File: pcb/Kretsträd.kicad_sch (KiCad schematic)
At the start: 56 parts, among them J1 Conn_01x02_Female, J2 Conn_01x02_Female, J3 Conn_01x02_Female, SW1 SW_PUSH, SW10 SW_PUSH, SW11 SW_PUSH, SW12 SW_PUSH, SW13 SW_PUSH, SW14 SW_PUSH, SW15 SW_PUSH, SW16 SW_PUSH, SW17 SW_PUSH, SW2 SW_PUSH, SW3 SW_PUSH, SW4 SW_PUSH, SW5 SW_PUSH, SW6 SW_PUSH, SW7 SW_PUSH, SW8 SW_PUSH, SW9 SW_PUSH, U1 SeeeduinoXIAO

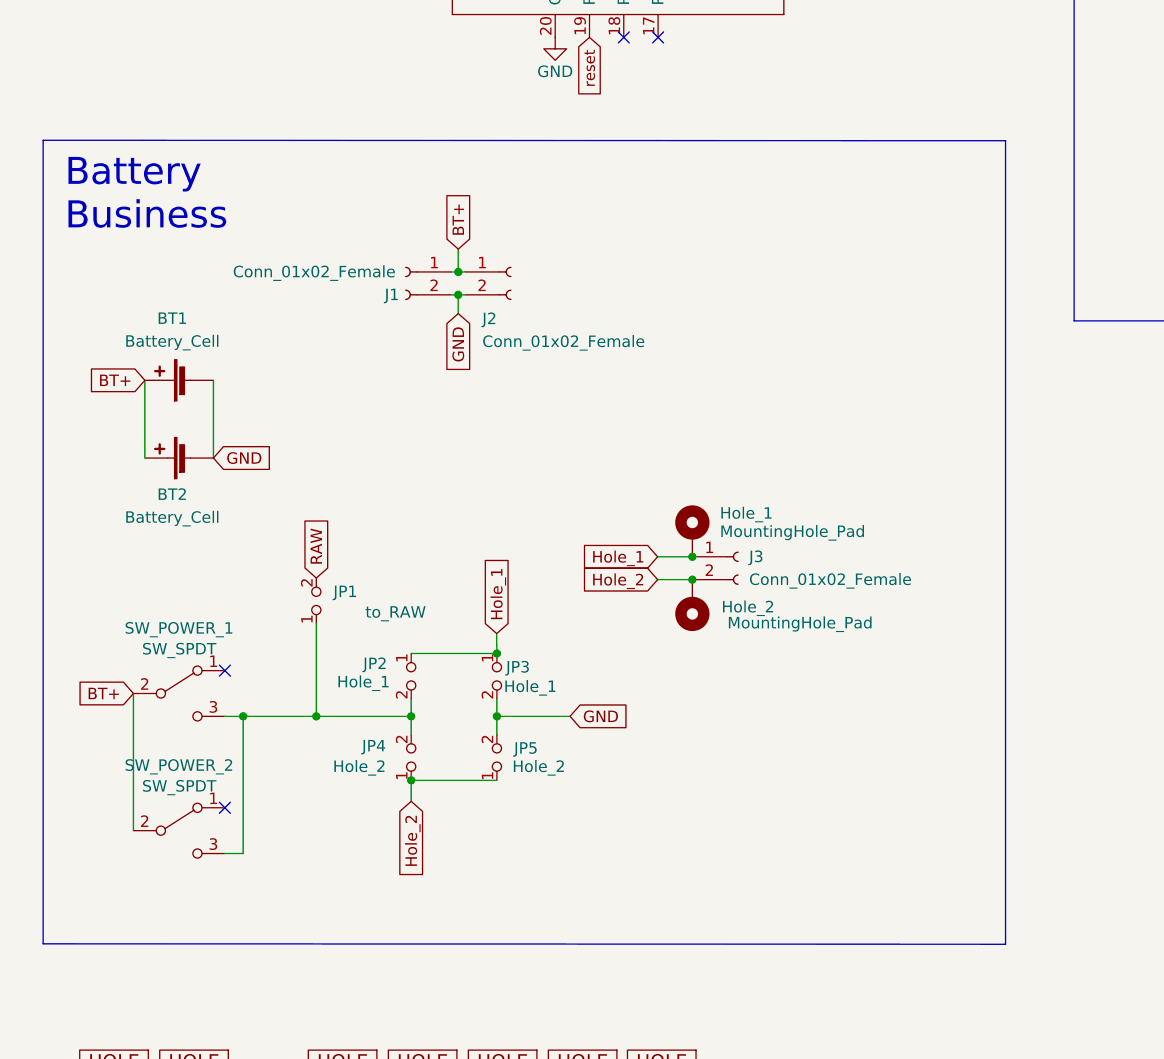
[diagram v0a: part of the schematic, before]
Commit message: Tones of changes.
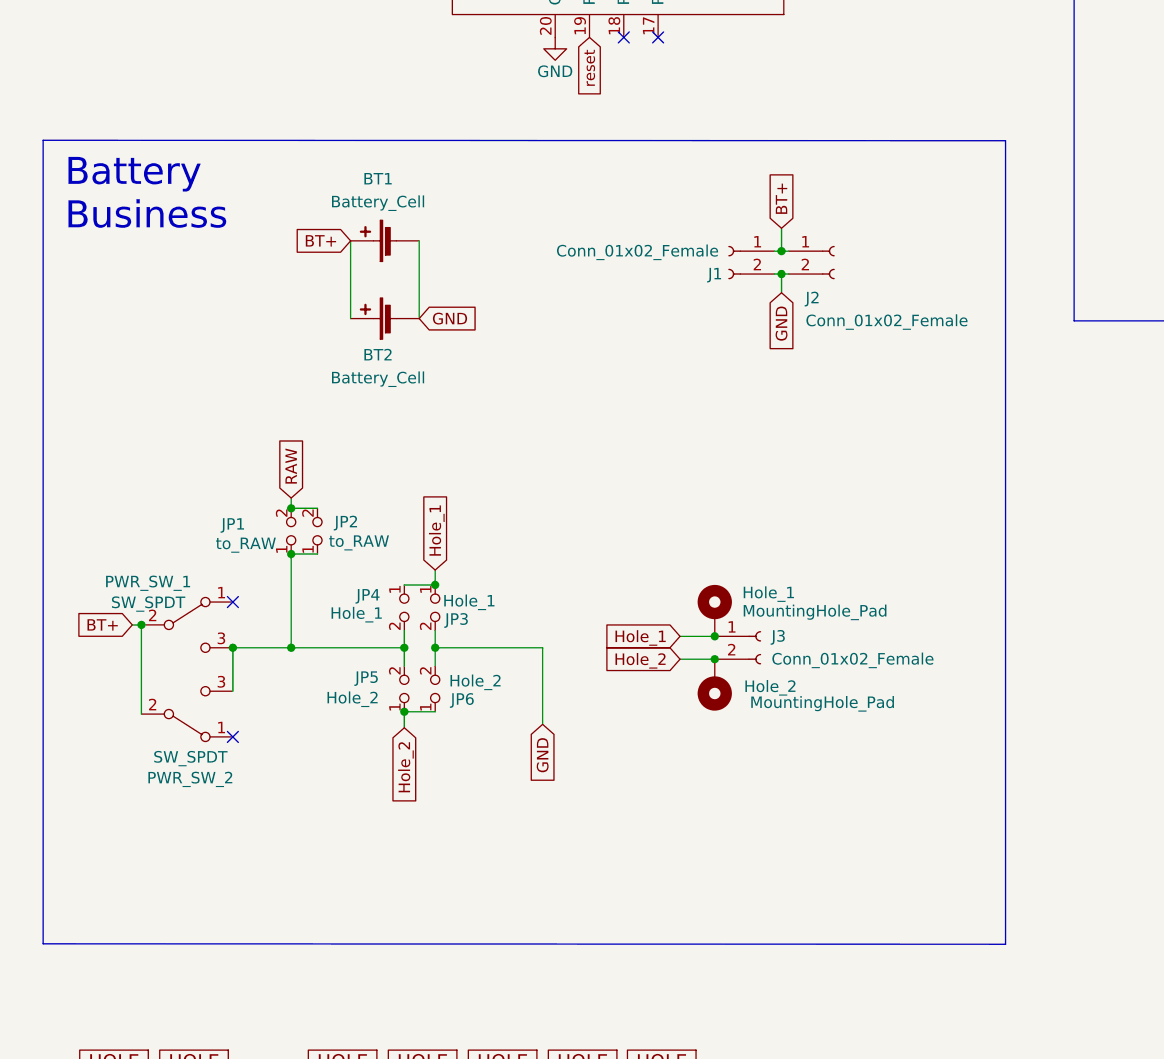
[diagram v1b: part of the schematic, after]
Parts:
- added JP1: to_RAW, Jumper:SolderJumper-2_P1.3mm_Open_RoundedPad1.0x1.5mm, symbol Device:Jumper_NO_Small
- D1, D10, D11, D12, D13, D14, D15, D16, D17, D2, D3, D4, D5, D6, D7, D8, D9: footprint jw_custom_footprint:D_SOD123_THT -> jw_custom_footprint:Diode_SOD123_THT_2
- JP2: renamed from JP1; footprint Jumper:SolderJumper-2_P1.3mm_Open_TrianglePad1.0x1.5mm -> Jumper:SolderJumper-2_P1.3mm_Open_RoundedPad1.0x1.5mm
- JP3: renamed from JP5; value Hole_2 -> Hole_1; footprint Jumper:SolderJumper-2_P1.3mm_Open_TrianglePad1.0x1.5mm -> Jumper:SolderJumper-2_P1.3mm_Open_RoundedPad1.0x1.5mm
- JP4: renamed from JP2; footprint Jumper:SolderJumper-2_P1.3mm_Open_TrianglePad1.0x1.5mm -> Jumper:SolderJumper-2_P1.3mm_Open_RoundedPad1.0x1.5mm
- JP5: renamed from JP4; footprint Jumper:SolderJumper-2_P1.3mm_Open_TrianglePad1.0x1.5mm -> Jumper:SolderJumper-2_P1.3mm_Open_RoundedPad1.0x1.5mm
- JP6: renamed from JP3; value Hole_1 -> Hole_2; footprint Jumper:SolderJumper-2_P1.3mm_Open_TrianglePad1.0x1.5mm -> Jumper:SolderJumper-2_P1.3mm_Open_RoundedPad1.0x1.5mm
- renumbered SW_POWER_1 to PWR_SW_1, SW_POWER_2 to PWR_SW_2
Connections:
- net Hole_1: now also JP3.1; no longer JP6.1
- net Hole_2: now also JP6.1; no longer JP3.1
- net RAW: now also JP1.2
- net at JP2.1, JP4.2, JP5.2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: now also JP1.1
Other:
- moved on the sheet: BT1, BT2, Hole_1, Hole_2, J1, J2, J3, JP2, JP3, JP4, JP5, JP6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
